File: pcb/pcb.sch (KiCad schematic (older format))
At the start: 38 parts, among them J1 USB_B_Mini, Q1 BSS138DW-7-F, SW1 PTS645Vx83, SW2 PTS645Vx83, SW3 PTS645Vx83, SW4 KMR2, U1 AP2112K-3.3, U2 MIC5225-1.8YM5, U3 CP2104, U5 ESP-12F

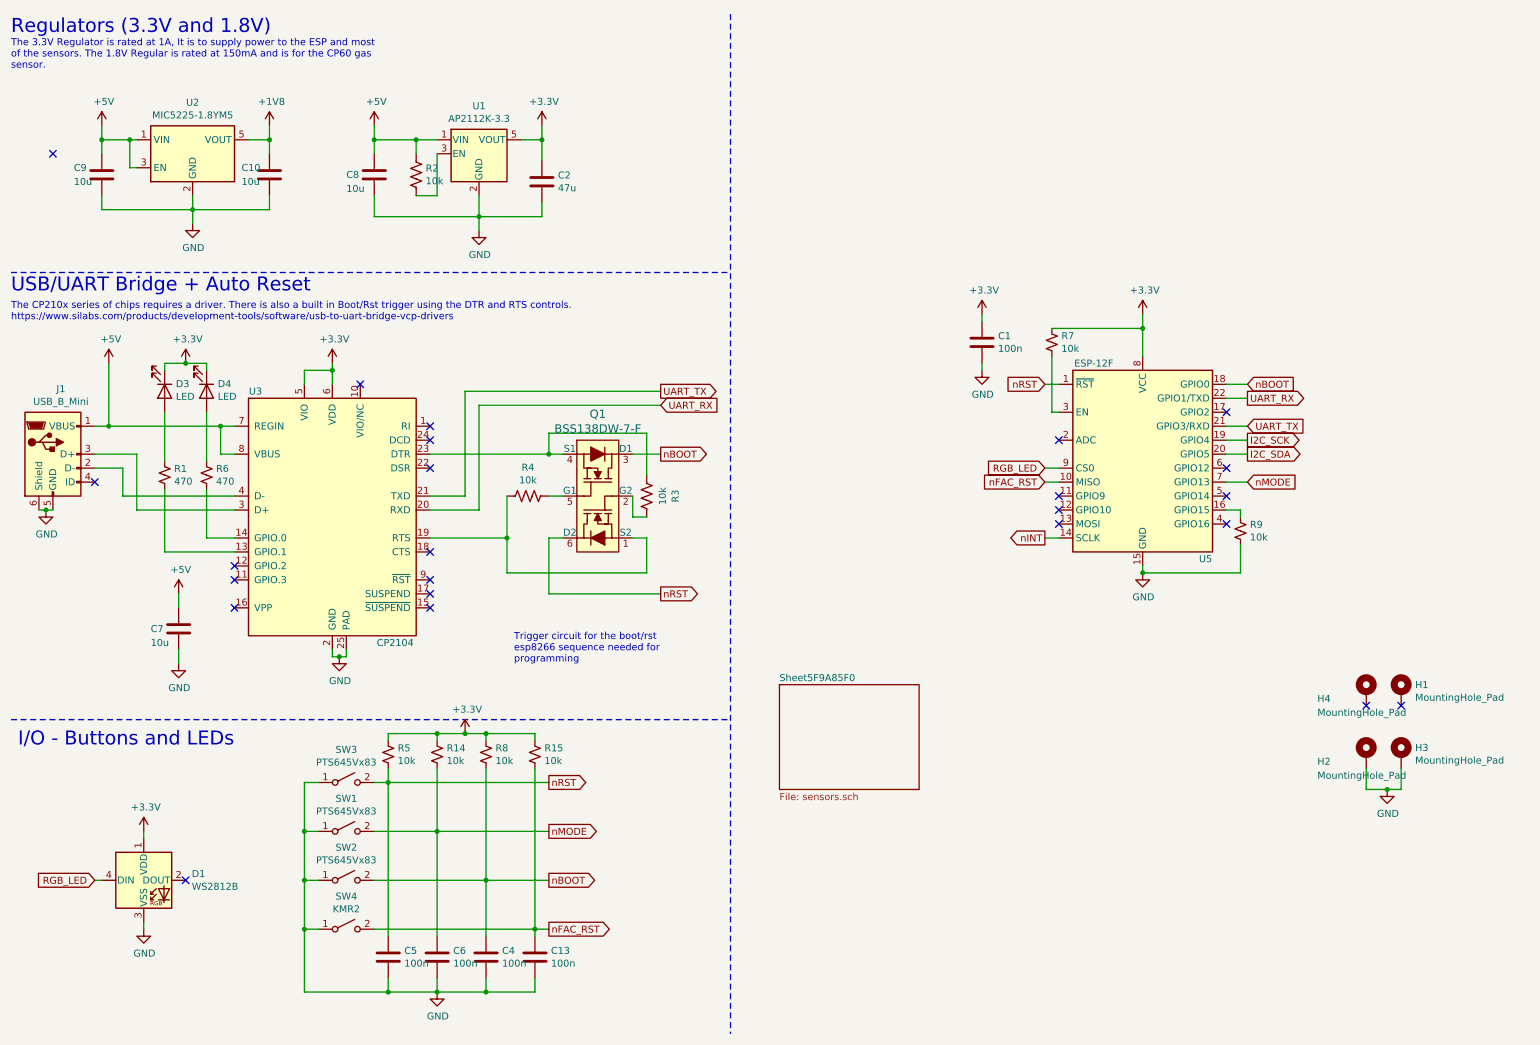
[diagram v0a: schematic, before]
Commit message: add gerbers for room monitor v1
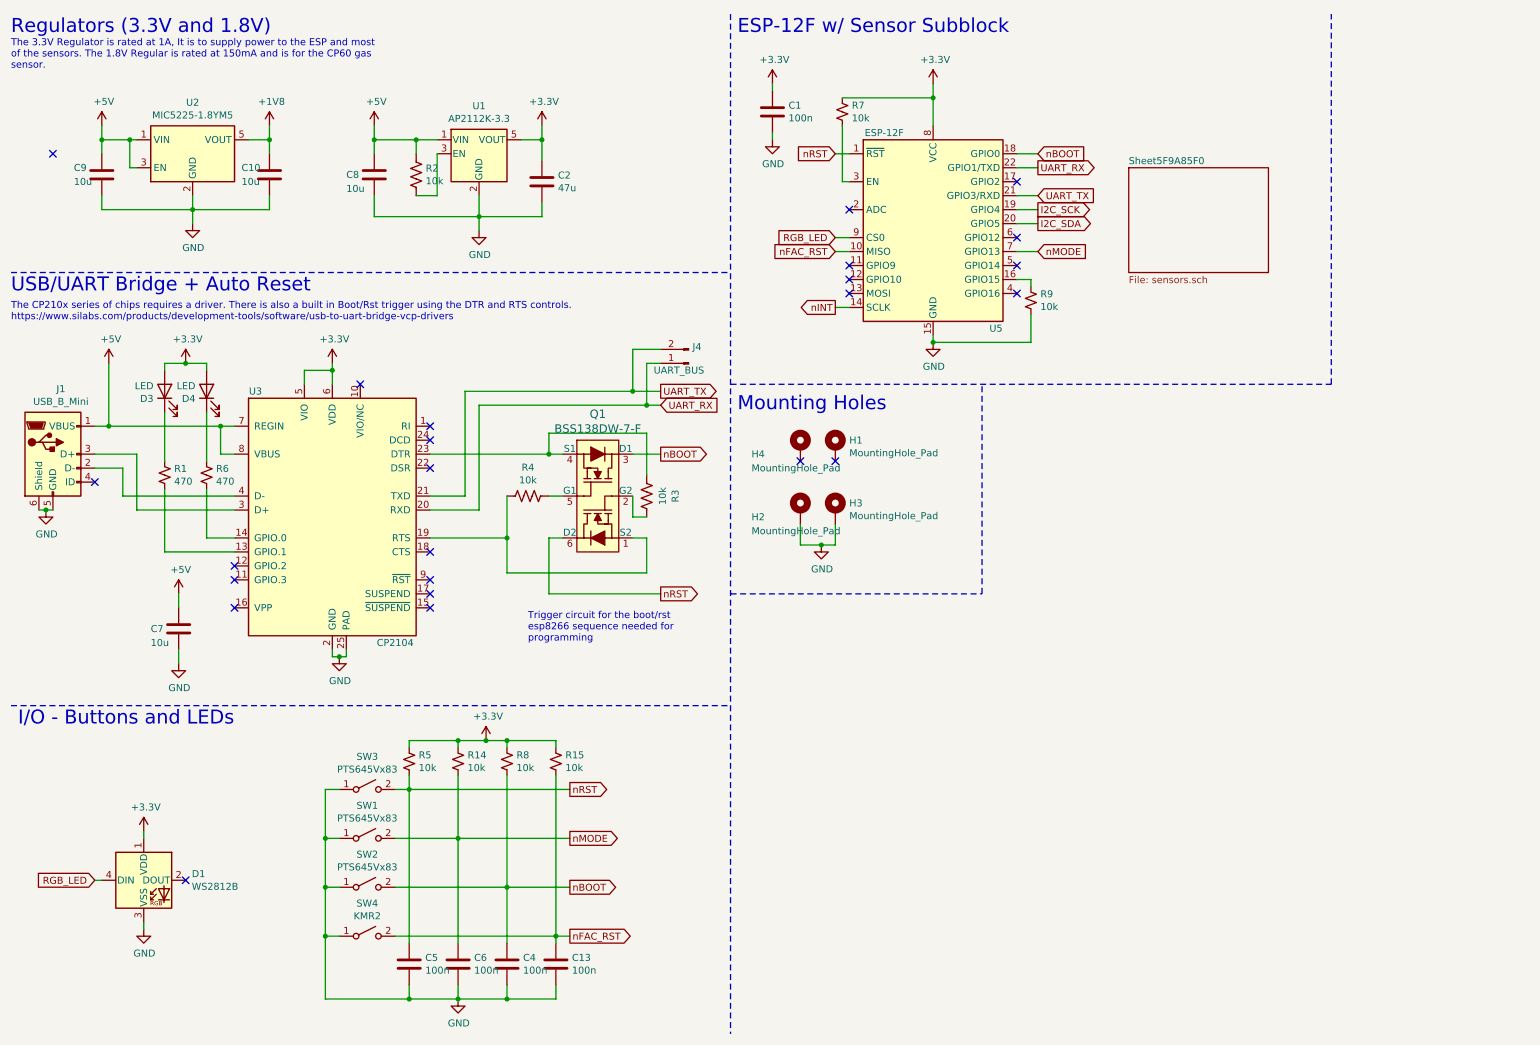
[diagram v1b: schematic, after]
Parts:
- added J4: UART_BUS, Connector_PinHeader_2.54mm:PinHeader_1x02_P2.54mm_Vertical, symbol Connector:Conn_01x02_Male
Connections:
- net +3V3: now also D3.2 (A), D4.2 (A); no longer D3.1 (K), D4.1 (K)
- net UART_RX: now also J4.1 (Pin_1)
- net UART_TX: now also J4.2 (Pin_2)
- net at R6.1: now also D4.1 (K); no longer D4.2 (A)
- net at R1.1: now also D3.1 (K); no longer D3.2 (A)
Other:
- note added: "ESP-12F w/ Sensor Subblock"
- note added: "Mounting Holes"
- moved on the sheet: C1, C13, C4, C5, C6, D3, D4, H1, H2, H3, H4, R14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

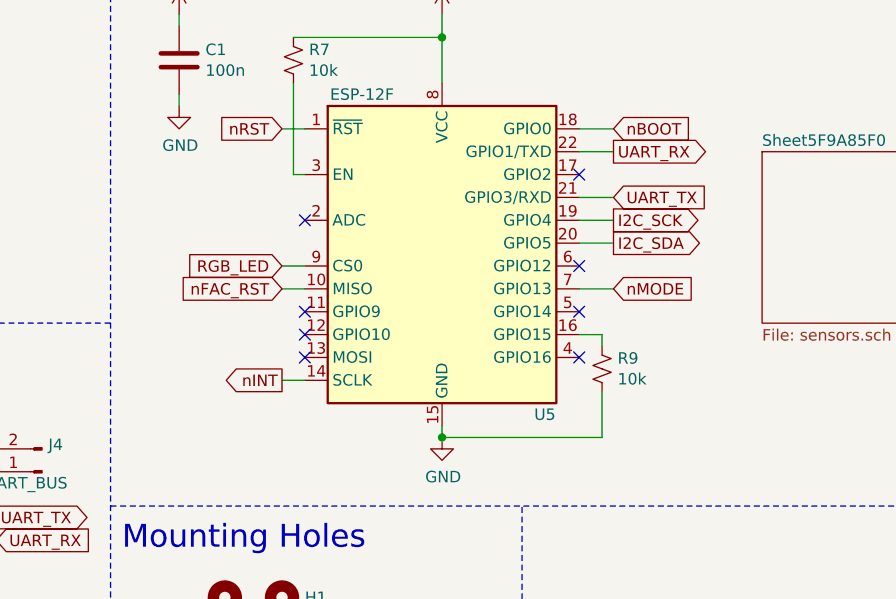
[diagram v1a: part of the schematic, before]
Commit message: WIP
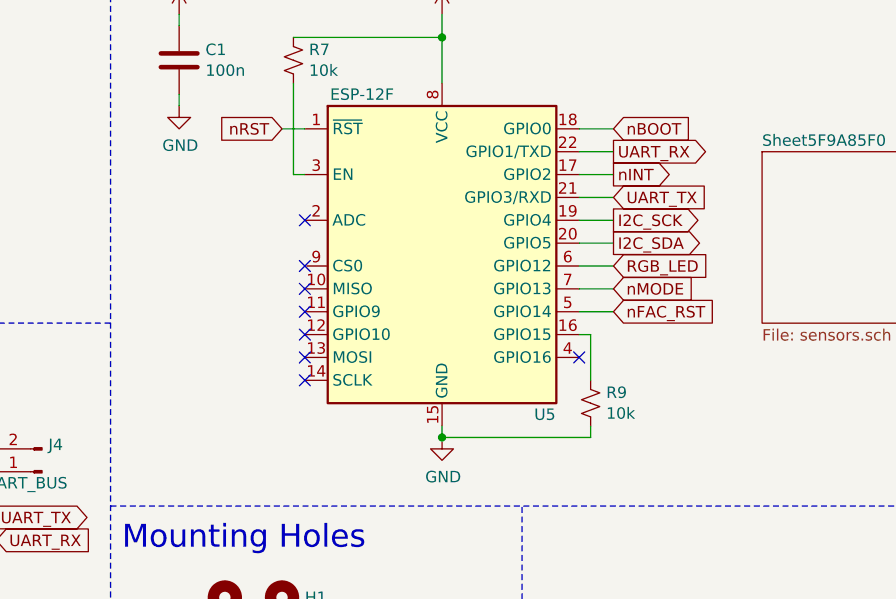
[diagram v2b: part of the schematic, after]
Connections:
- net RGB_LED: now also U5.6 (GPIO12); no longer U5.9 (CS0)
- net nFAC_RST: now also U5.5 (GPIO14); no longer U5.10 (MISO)
- net nINT: now also U5.17 (GPIO2); no longer U5.14 (SCLK)
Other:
- moved on the sheet: R9
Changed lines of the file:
@@
 	6450 1700 6500 1700
 Wire Wire Line
-	7700 2400 7800 2400
+	7700 2400 7750 2400
 Text GLabel 7850 1900 2    50   Output ~ 0
 I2C_SCK
@@
 NoConn ~ 6500 2300
 NoConn ~ 6500 2400
-NoConn ~ 7700 2500
-NoConn ~ 7700 2300
-NoConn ~ 7700 2100
 Wire Notes Line
 	5650 500  5650 7800
-Text GLabel 6400 2100 0    50   Input ~ 0
-RGB_LED
 $Comp
 L Device:R_US R2
@@
 NoConn ~ 1750 6700
 NoConn ~ 3000 3150
-Text GLabel 6400 2600 0    50   Output ~ 0
+Text GLabel 7850 1700 2    50   Output ~ 0
 nINT
-Wire Wire Line
-	6400 2600 6500 2600
 $Comp
 L dk_Transistors-FETs-MOSFETs-Arrays:BSS138DW-7-F Q1
@@
 L Device:R_Small_US R9
 U 1 1 5F341E1A
-P 7800 2550
-F 0 "R9" H 7868 2596 50  0000 L CNN
-F 1 "10k" H 7868 2505 50  0000 L CNN
-F 2 "Resistor_SMD:R_0603_1608Metric" H 7800 2550 50  0001 C CNN
-F 3 "~" H 7800 2550 50  0001 C CNN
-	1    7800 2550
-	1    0    0    -1
-$EndComp
-Wire Wire Line
-	7800 2400 7800 2450
+P 7750 2700
+F 0 "R9" H 7818 2746 50  0000 L CNN
+F 1 "10k" H 7818 2655 50  0000 L CNN
+F 2 "Resistor_SMD:R_0603_1608Metric" H 7750 2700 50  0001 C CNN
+F 3 "~" H 7750 2700 50  0001 C CNN
+	1    7750 2700
+	1    0    0    -1
+$EndComp
+Wire Wire Line
+	7750 2400 7750 2600
 Wire Wire Line
 	6450 1300 6450 1700
@@
 	7100 1100 7100 1000
 Wire Wire Line
-	7100 2850 7800 2850
+	7100 2850 7750 2850
 Connection ~ 7100 2850
 Wire Wire Line
-	7800 2650 7800 2850
-Wire Wire Line
-	6400 2100 6500 2100
+	7750 2800 7750 2850
 NoConn ~ 6500 2500
-Text GLabel 6400 2200 0    50   Input ~ 0
+Text GLabel 7850 2300 2    50   Input ~ 0
 nFAC_RST
 Wire Wire Line
-	6400 2200 6500 2200
-NoConn ~ 7700 1700
+	7850 2300 7700 2300
 Text Notes 5700 650  0    100  ~ 0
 ESP-12F w/ Sensor Subblock
@@
 Wire Wire Line
 	3500 3650 4350 3650
+Text GLabel 7850 2100 2    50   Input ~ 0
+RGB_LED
+Wire Wire Line
+	7700 2100 7850 2100
+Wire Wire Line
+	7700 1700 7850 1700
+NoConn ~ 7700 2500
+NoConn ~ 6500 2100
+NoConn ~ 6500 2200
+NoConn ~ 6500 2600
 $EndSCHEMATC
